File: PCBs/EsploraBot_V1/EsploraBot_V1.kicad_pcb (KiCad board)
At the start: 2 copper layers, 100 x 82 mm, 17 parts, among them J1 HMC5883L, J2 VL53L0X_IZQ, J3 VL53L0X_DER, J4 HC-SR04, J5 Batería, J6 MotorIzq, J7 MotorDer, SW1 SW_SPDT, U1 ESP32-DEVKIT-V1, U2 TB6612FNG_1, U3 module_mpu6050, U4 LM2596

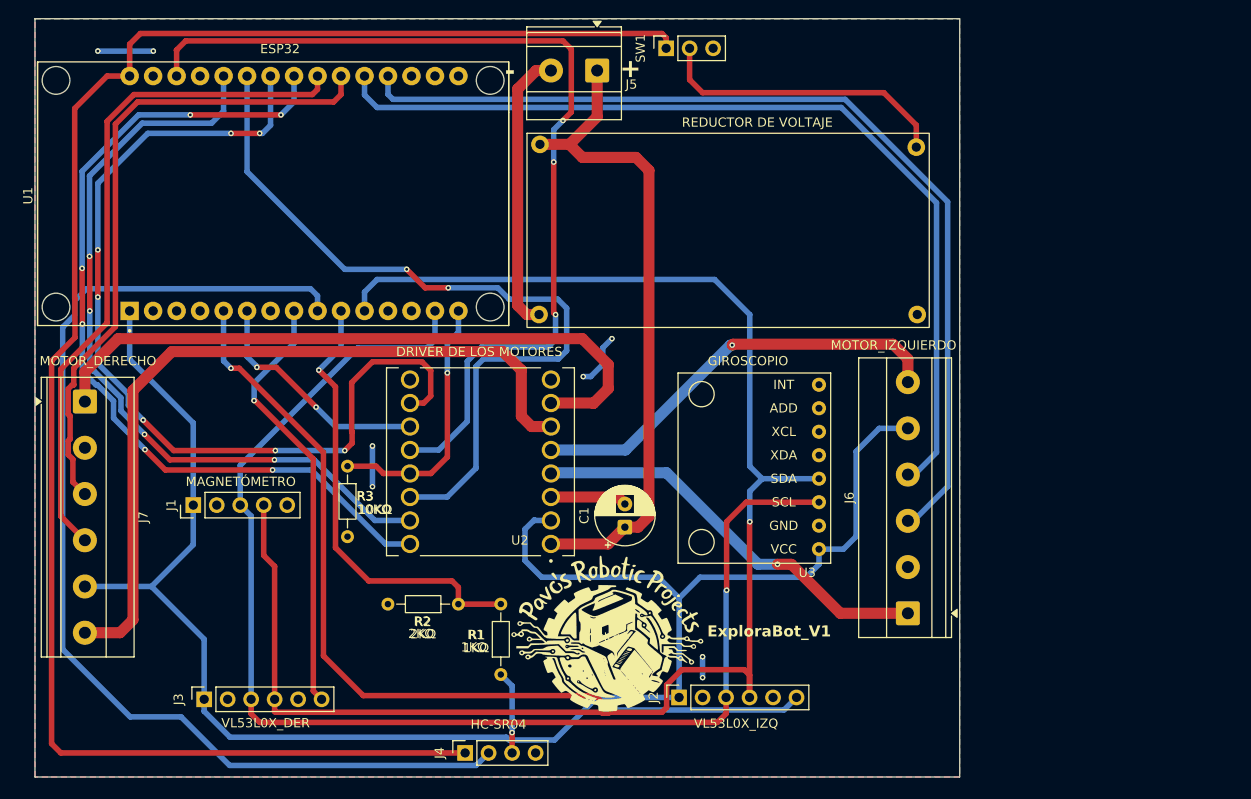
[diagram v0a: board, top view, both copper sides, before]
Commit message: fix: Se realizaron algunos ajuste esteticos en el esquematico y PCB
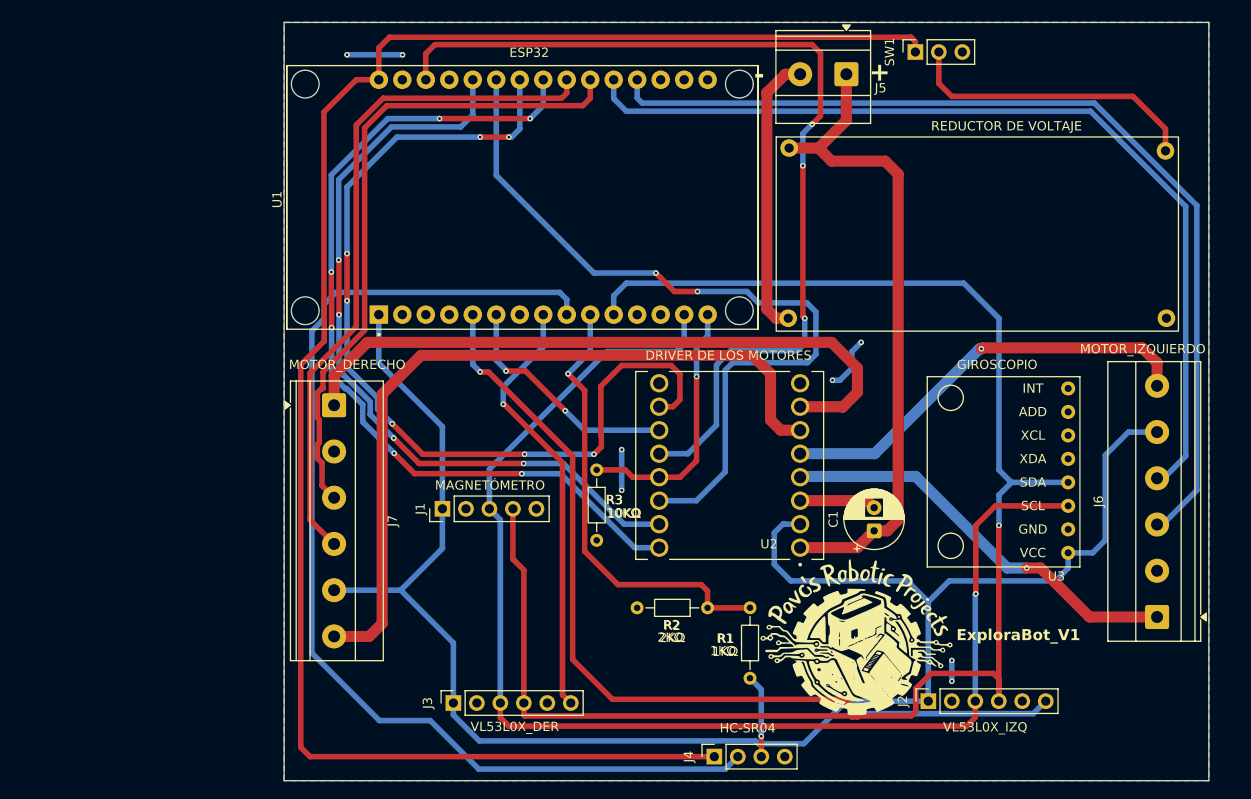
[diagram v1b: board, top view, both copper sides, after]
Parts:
- moved U1 27.0 mm to (77.3, 35.1)
- moved G*** 27.0 mm to (113.5, 83.4)
- moved J1 27.0 mm to (68.7, 68.8)
- moved J7 27.0 mm to (57.0, 57.6)
- moved R1 27.0 mm to (101.9, 87.1)
- moved R2 27.0 mm to (97.3, 79.5)
- moved SW1 27.0 mm to (119.8, 19.4)
- moved U2 27.0 mm to (99.7, 64.1)
- moved U3 27.0 mm to (136.3, 55.8)
- moved U4 27.0 mm to (103.1, 51.2)
- moved J3 27.0 mm to (69.8, 89.8)
- moved R3 27.0 mm to (85.3, 64.6)
- moved C1 27.0 mm to (115.3, 71.2)
- moved J2 27.0 mm to (121.2, 89.6)
- moved J4 27.0 mm to (98.1, 95.6)
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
